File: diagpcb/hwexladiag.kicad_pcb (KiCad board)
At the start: 2 copper layers, 20 x 30 mm, 16 parts, among them J1 PINHEADER, Q1 2N7002, Q2 2N7002, SW1 SW_Push, U1 HC05, U2 HT7533-1

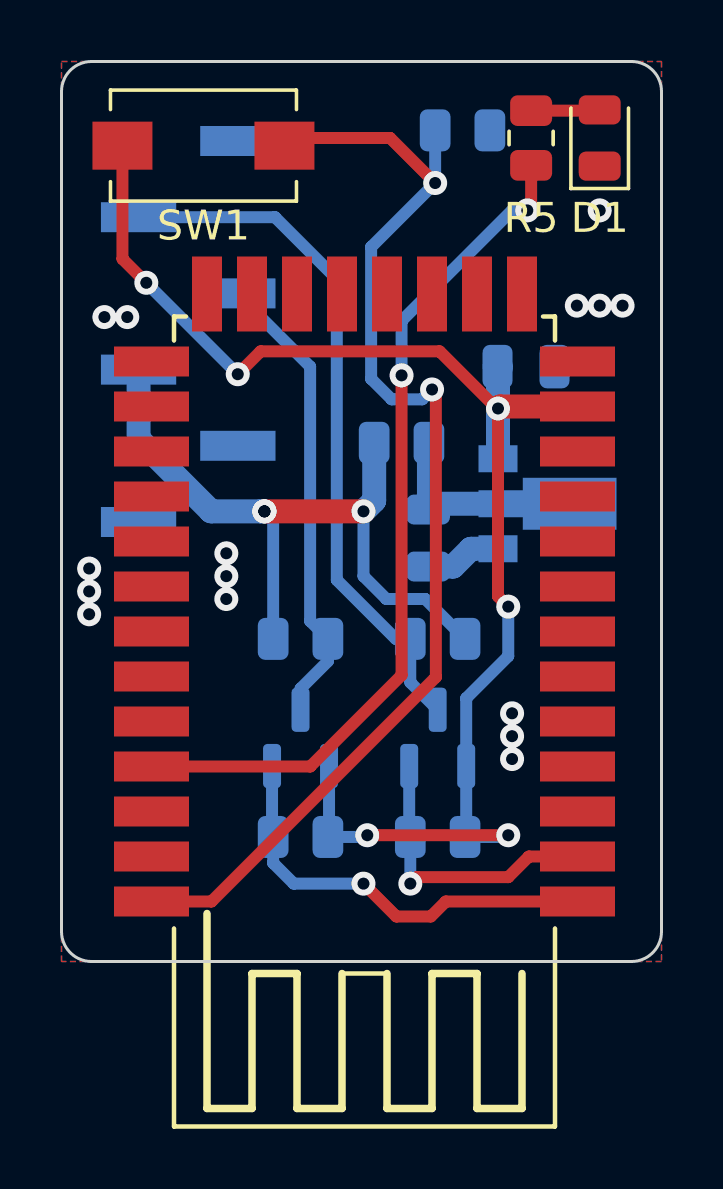
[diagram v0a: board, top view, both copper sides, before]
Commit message: Use smaller HC05 footprint.
Make the PCB smaller by 2.8 mm.
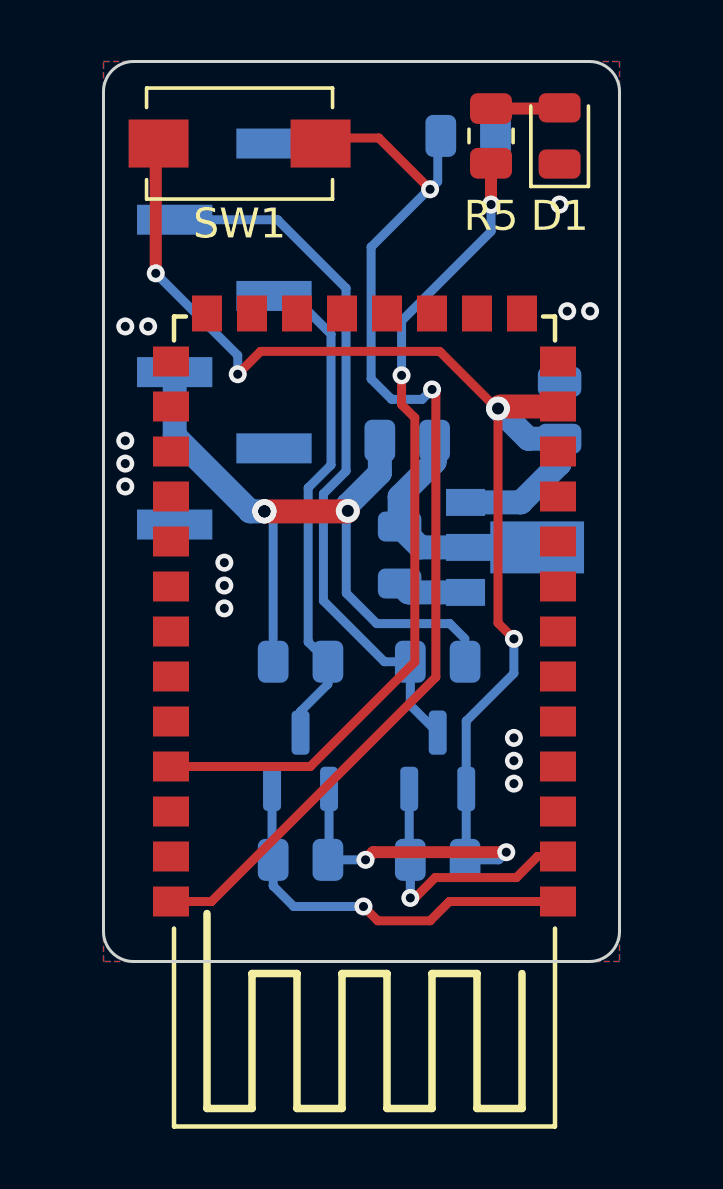
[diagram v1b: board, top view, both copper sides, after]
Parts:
- moved C2 1.84 mm to (153.6, 91.6), turned to 90 degrees
- moved U2 1.81 mm to (152.4, 96.2)
- moved D1 1.34 mm to (153.6, 82.5)
- moved R5 1.34 mm to (151.3, 82.5)
- moved J1 1.21 mm to (142.4, 89.1)
- moved SW1 1.21 mm to (142.9, 82.7)
- moved C1 1.11 mm to (148.3, 96.5)
- moved Q1 0.76 mm to (149.5, 103.3)
- moved Q2 0.76 mm to (145.0, 103.3)
- moved R1 0.76 mm to (149.5, 100.0)
- moved R2 0.76 mm to (149.5, 106.6)
- moved R3 0.76 mm to (145.0, 100.0)
- moved R4 0.76 mm to (145.0, 106.6)
- moved R7 0.26 mm to (150.6, 82.5)
- moved R6 0.20 mm to (148.5, 92.6)
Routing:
- net +3V3: track 49.6 -> 53.6 mm
- net Net-(U1-PIO11): track 39.6 -> 37.5 mm
- net Net-(U2-VIN): track 4.73 -> 5.92 mm
- net Net-(U1-PIO8): track 28.7 -> 27.6 mm
- net /HCTX: track 14.3 -> 13.5 mm
- net /HCRX: track 9.88 -> 9.14 mm
- net /wexlaRxD: track 15.5 -> 16.2 mm
- net +5V: track 24.0 -> 23.5 mm
- net GND: track 2.57 -> 2.32 mm, vias 15 -> 14
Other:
- board size 20 x 30 mm -> 17.2 x 30 mm
- board text added: "JH 2024 v1.1"
- board text removed: "JH 2023 v1.0"
